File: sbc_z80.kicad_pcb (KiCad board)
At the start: 4 copper layers, 101.6 x 50.8 mm, 61 parts, among them J1 RC80 Bus, J2 UPDI TTL, J3 Conn_02x12_Odd_Even, J4 Conn_01x06, J5 Conn_01x06, J6 Conn_01x10, J7 AVR-JTAG-10, SW1 SW_Push, U1 CPU - Z84C0010AEG, U10 74HC3G34DP,125, U11 MIC5356-SGYMME, U12 MIC811LUY, U2 Si5351A-B-GT, U3 SRAM - IS62C5128BL-45TLI, U4 ROM - GLS29EE512, U5 ATtiny1614-SS, U6 SIO/3 - Z84C4310AEG, U7 CPLD - EPM7032STC44, U8 CTC - Z84C3010AEG, U9 PIO - Z84C2010AEG, Y1 25MHZ 8PF

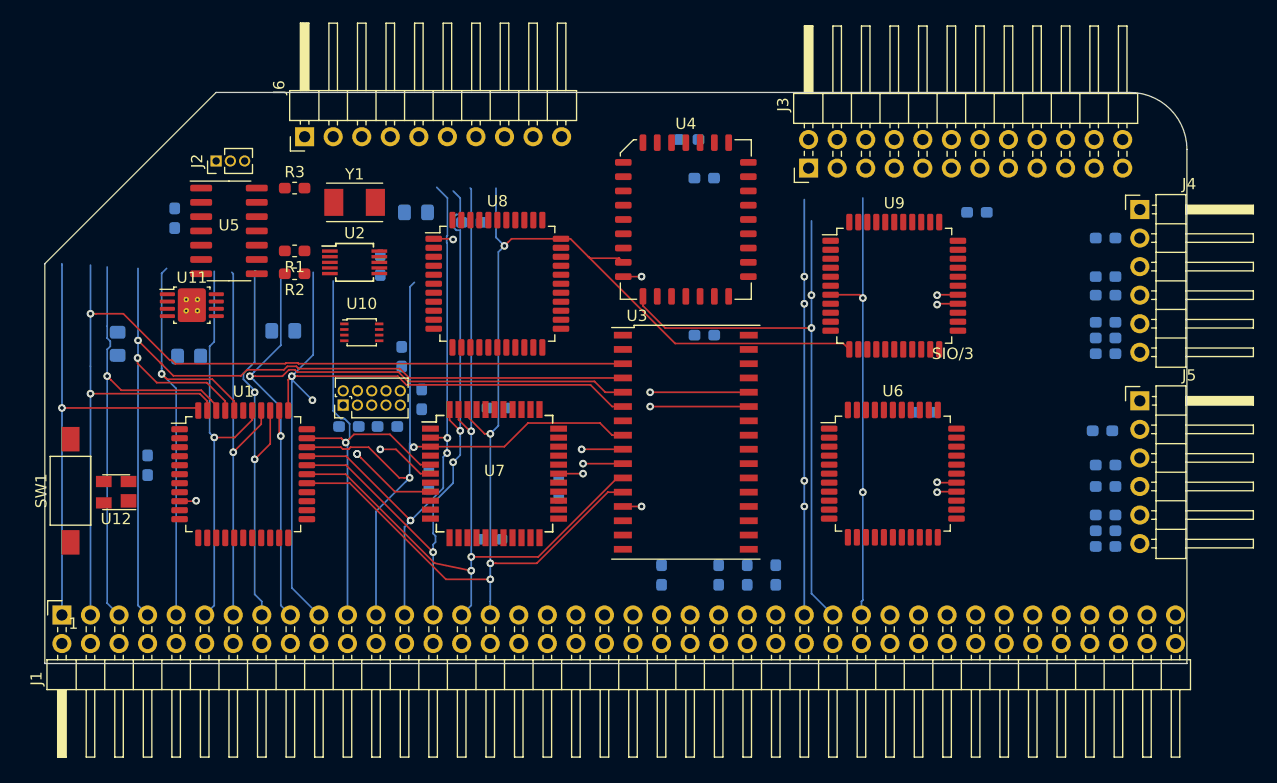
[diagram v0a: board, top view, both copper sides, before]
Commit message: changed part layouts
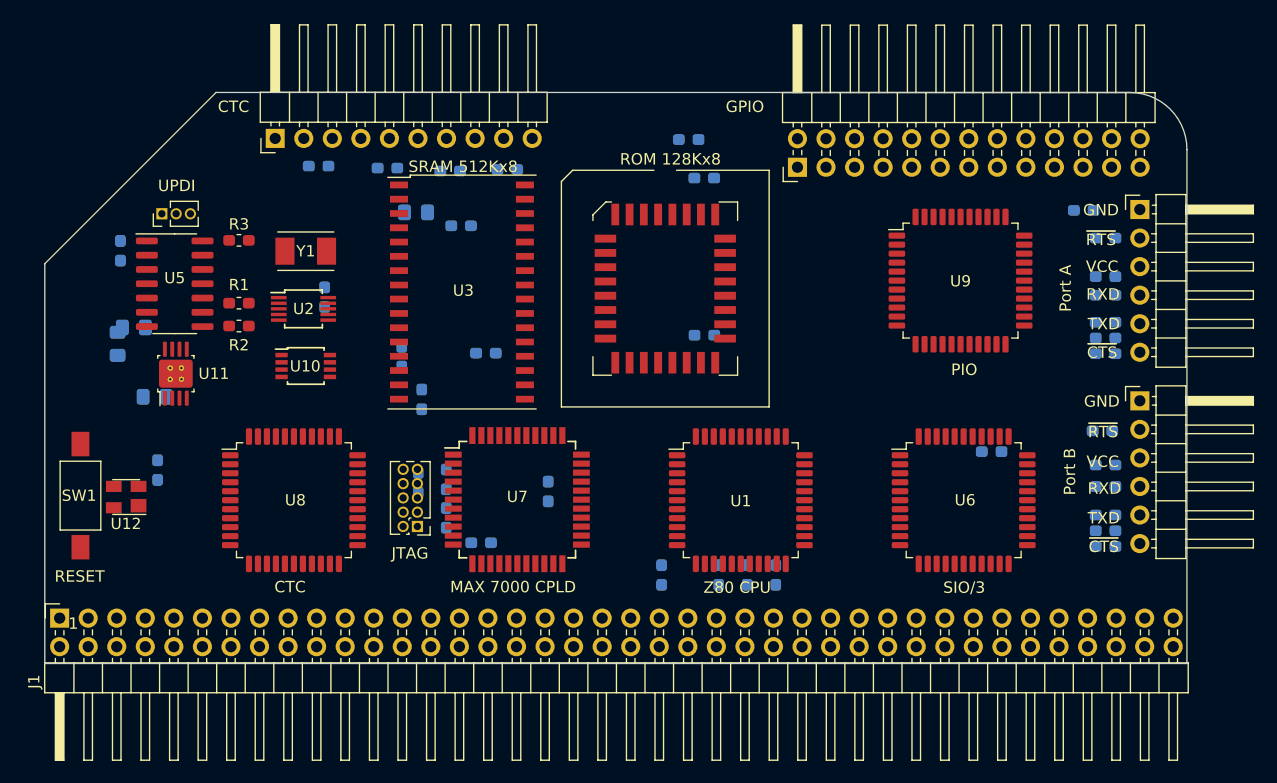
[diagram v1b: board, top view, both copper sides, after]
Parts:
- added R25: 10K, Resistor_SMD:R_0603_1608Metric_Pad1.05x0.95mm_HandSolder, B.Cu at (99.8, 83.3)
- added R26: 10K, Resistor_SMD:R_0603_1608Metric_Pad1.05x0.95mm_HandSolder, B.Cu at (105.9, 83.4)
- added R27: 10K, Resistor_SMD:R_0603_1608Metric_Pad1.05x0.95mm_HandSolder, B.Cu at (111.5, 83.7)
- added R28: 10K, Resistor_SMD:R_0603_1608Metric_Pad1.05x0.95mm_HandSolder, B.Cu at (116.6, 83.6)
- J3: value Conn_02x12_Odd_Even -> PIO Header; footprint Connector_PinHeader_2.54mm:PinHeader_2x12_P2.54mm_Horizontal -> Connector_PinHeader_2.54mm:PinHeader_2x13_P2.54mm_Horizontal
- J6: value Conn_01x10 -> CTC Header
- R10, R11, R12, R13, R16, R17, R18, R19: value 2.2K -> 2K2
- U10: value 74HC3G34DP,125 -> 74HC3G04DP,125; footprint Package_SO:VSSOP-8_2.4x2.1mm_P0.5mm -> Package_SO:TSSOP-8_3x3mm_P0.65mm
- U4: value ROM - GLS29EE512 -> GLS29EE010; footprint Package_LCC:PLCC-32_11.4x14.0mm_P1.27mm -> Package_LCC:PLCC-32_SMD-Socket
- moved U1 44.3 mm to (137.4, 113.0)
- moved U8 26.4 mm to (97.6, 113.0)
- moved U3 24.0 mm to (112.5, 94.5)
- moved C4 13.3 mm to (83.4, 97.6), turned to 180 degrees
- moved J7 12.7 mm to (108.6, 115.3), turned to 180 degrees
- moved R23 11.9 mm to (111.2, 114.6), turned to 90 degrees
- moved C12 9.50 mm to (167.9, 87.2)
- moved R22 7.03 mm to (111.2, 111.1), turned to 270 degrees
- moved C11 6.94 mm to (159.7, 108.7)
- moved R2 6.79 mm to (92.7, 97.5)
- moved R3 6.79 mm to (92.7, 89.9)
- moved R1 6.79 mm to (92.7, 95.5)
- moved J2 6.74 mm to (85.9, 87.5)
- moved U5 6.74 mm to (87.0, 93.7)
- moved U6 6.73 mm to (157.2, 113.0)
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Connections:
- C10 pad 1: +5V -> Net-(C10-Pad1)
- C11 pad 1: +5V -> Net-(C10-Pad1)
- C12 pad 1: +5V -> Net-(C10-Pad1)
- C13 pad 1: +5V -> Net-(C10-Pad1)
- C14 pad 1: +5V -> Net-(C10-Pad1)
- C5 pad 1: +5V -> Net-(C10-Pad1)
- C6 pad 1: +5V -> Net-(C10-Pad1)
- C7 pad 1: +5V -> Net-(C10-Pad1)
- C8 pad 1: +5V -> Net-(C10-Pad1)
- C9 pad 1: +5V -> Net-(C10-Pad1)
- J1 pad 54: (no net) -> /A18
- J1 pad 55: (no net) -> /A17
- J1 pad 56: (no net) -> /A16
- J3 pad 1: (no net) -> +5V
- J3 pad 10: (no net) -> /PB2
- J3 pad 11: (no net) -> /PA4
- J3 pad 12: (no net) -> /PB3
- J3 pad 13: (no net) -> /PA5
- J3 pad 14: (no net) -> /PB4
- J3 pad 15: (no net) -> /PA6
- J3 pad 16: (no net) -> /PB5
- J3 pad 17: (no net) -> /PA7
- J3 pad 18: (no net) -> /PB6
- J3 pad 19: (no net) -> /ARDY
- J3 pad 2: (no net) -> GND
- J3 pad 20: (no net) -> /PB7
- J3 pad 21: (no net) -> /~ASTB
- J3 pad 22: (no net) -> /BRDY
- J3 pad 23: (no net) -> GND
- J3 pad 24: (no net) -> /~BSTB
- J3 pad 3: (no net) -> /PA0
- J3 pad 4: (no net) -> GND
- J3 pad 5: (no net) -> /PA1
- J3 pad 6: (no net) -> /PB0
- J3 pad 7: (no net) -> /PA2
- J3 pad 8: (no net) -> /PB1
- J3 pad 9: (no net) -> /PA3
- J6 pad 1: (no net) -> +5V
- J6 pad 10: (no net) -> GND
- J6 pad 2: (no net) -> /CT0
- J6 pad 3: (no net) -> /ZT0
- J6 pad 4: (no net) -> /CT1
- J6 pad 5: (no net) -> /ZT1
- J6 pad 6: (no net) -> /CT2
- J6 pad 7: (no net) -> /ZT2
- J6 pad 8: (no net) -> /CT3
- U3 pad 1: /BANK2 -> /A17
- U3 pad 2: /BANK1 -> /A16
- U3 pad 30: /BANK3 -> /A18
- U4 pad 2: Net-(U4-Pad1) -> /A16
- U7 pad 20: /BANK3 -> /A18
- U7 pad 21: /BANK2 -> /A17
- U7 pad 22: /BANK1 -> /A16
- U8 pad 16: (no net) -> /ZT0
- U8 pad 18: (no net) -> /ZT1
- U8 pad 19: (no net) -> /ZT2
- U8 pad 32: (no net) -> /~RESET
- U8 pad 36: (no net) -> /CT3
- U8 pad 37: (no net) -> /CT2
- U8 pad 40: (no net) -> /CT1
- U8 pad 41: (no net) -> /CT0
- U9 pad 13: (no net) -> /PA7
- U9 pad 14: (no net) -> /PA6
- U9 pad 15: (no net) -> /PA5
- U9 pad 16: (no net) -> /PA4
- U9 pad 19: (no net) -> /PA3
- U9 pad 20: (no net) -> /PA2
- U9 pad 21: (no net) -> /PA1
- U9 pad 22: (no net) -> /PA0
- U9 pad 23: (no net) -> /~ASTB
- U9 pad 24: (no net) -> /~BSTB
- U9 pad 25: (no net) -> /ARDY
- U9 pad 29: (no net) -> /BRDY
- U9 pad 35: (no net) -> /PB0
- U9 pad 36: (no net) -> /PB1
- U9 pad 37: (no net) -> /PB2
- U9 pad 38: (no net) -> /PB3
- U9 pad 40: (no net) -> /PB4
- U9 pad 41: (no net) -> /PB5
- U9 pad 42: (no net) -> /PB6
- U9 pad 43: (no net) -> /PB7
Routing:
- net /D0: track 175.7 -> 0.00 mm, vias 11 -> 0
- net /A0: track 114.7 -> 0.00 mm, vias 4 -> 0
- net /A13: track 100.5 -> 0.00 mm, vias 2 -> 0
- net /A14: track 91.9 -> 0.00 mm, vias 2 -> 0
- net /A12: track 87.7 -> 0.00 mm, vias 2 -> 0
- net /A7: track 85.1 -> 0.00 mm, vias 4 -> 0
- net /A6: track 82.1 -> 0.00 mm, vias 3 -> 0
- net /A8: track 81.7 -> 0.00 mm, vias 3 -> 0
- net /A1: track 75.2 -> 0.00 mm, vias 3 -> 0
- net /A2: track 71.9 -> 0.00 mm, vias 4 -> 0
- net /A3: track 68.9 -> 0.00 mm, vias 4 -> 0
- net /D1: track 65.8 -> 0.00 mm, vias 3 -> 0
- net /A4: track 61.8 -> 0.00 mm, vias 2 -> 0
- net /D2: track 48.5 -> 0.00 mm, vias 3 -> 0
- net /A15: track 43.5 -> 0.00 mm, vias 1 -> 0
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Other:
- board text added: "CTC"
- board text added: "GND"
- board text added: "GPIO"
- board text added: "JTAG"
- board text added: "MAX 7000 CPLD"
- board text added: "PIO"
- board text added: "Port A"
- board text added: "Port B"
- board text added: "RESET"
- board text added: "ROM 128Kx8"
- board text added: "RXD"
- board text added: "SRAM 512Kx8"
- board text added: "TXD"
- board text added: "UPDI"
- board text added: "VCC"
- board text added: "Z80 CPU"
- board text added: "~CTS"
- board text added: "~RTS"
